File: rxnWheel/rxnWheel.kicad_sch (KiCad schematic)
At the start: 14 parts, among them IC1 TB9061AFNG,EL

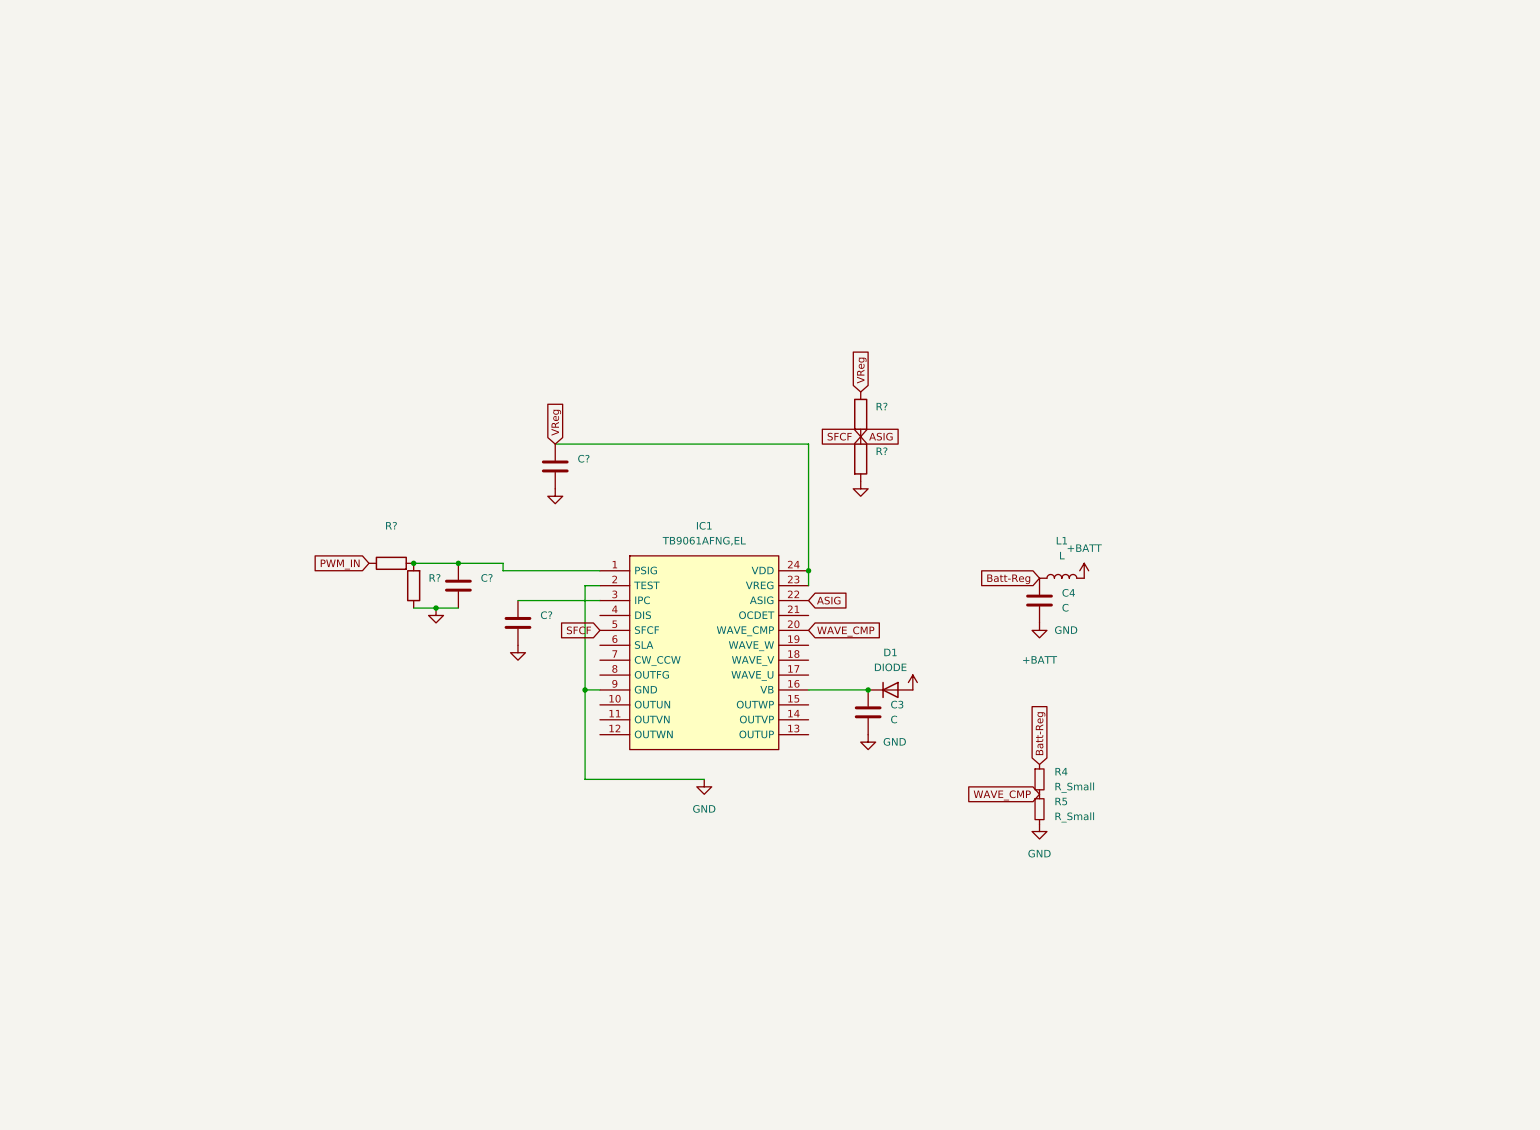
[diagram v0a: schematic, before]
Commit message: .
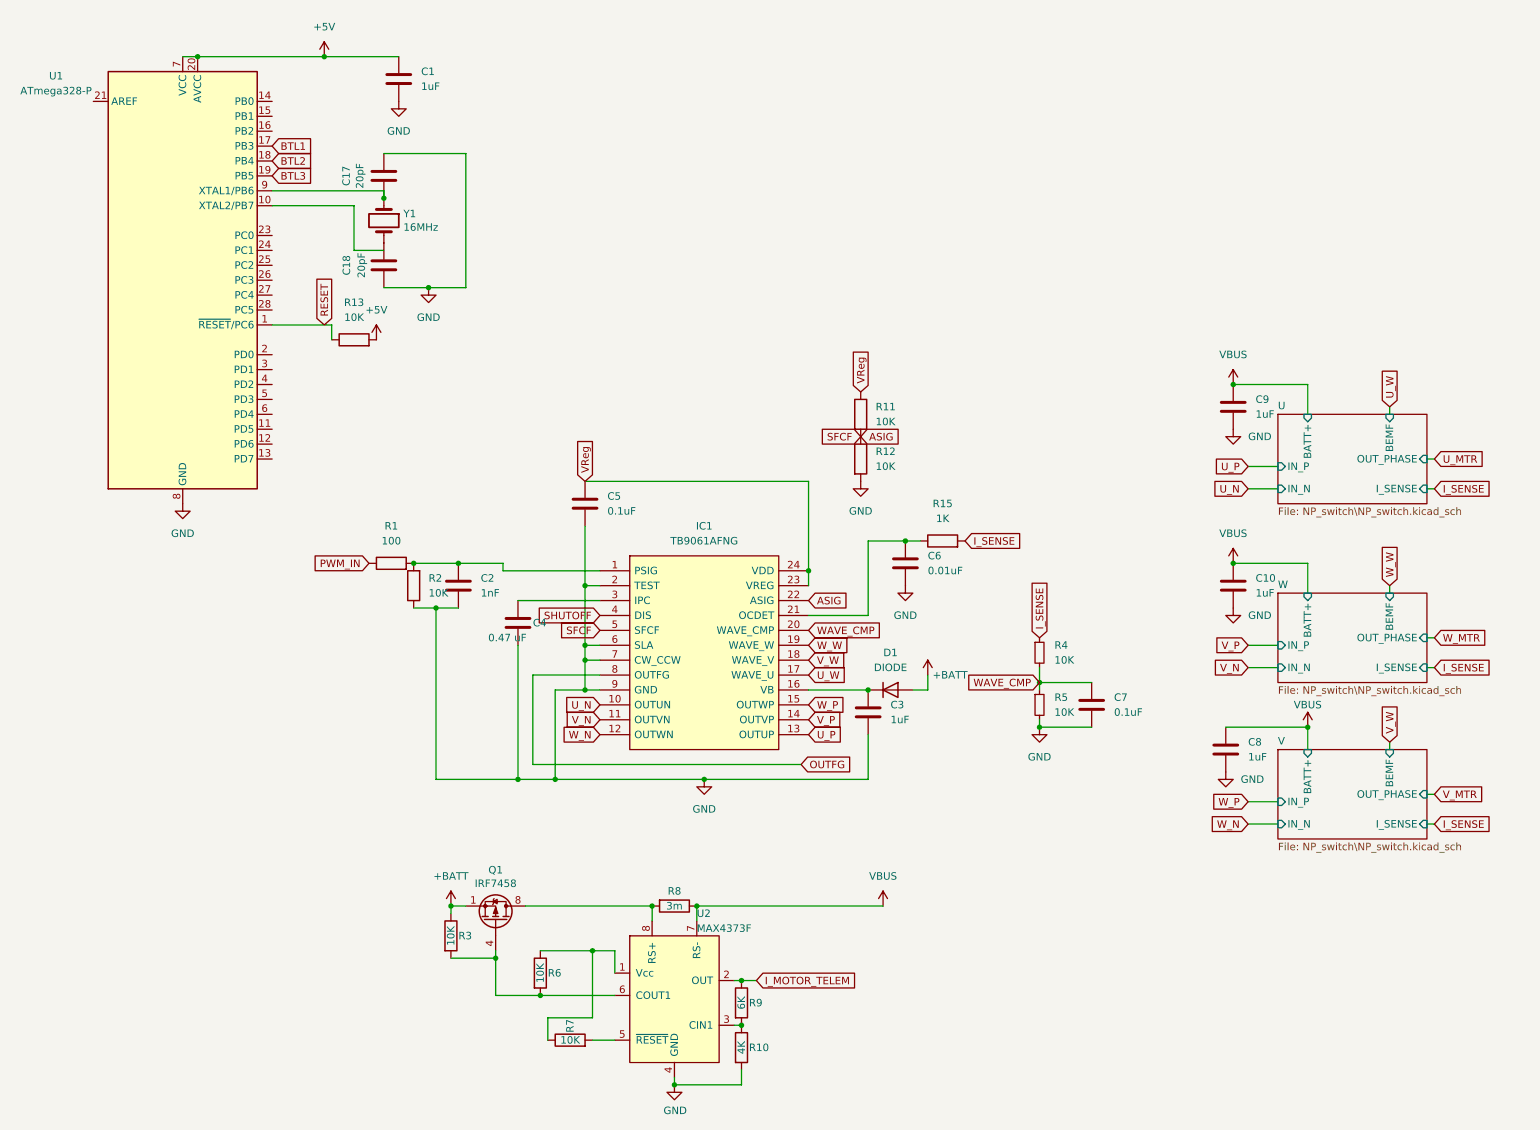
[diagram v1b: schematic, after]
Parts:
- removed C4: C, symbol Device:C
- removed L1: L, symbol Device:L
- added C1, C10, C8, C9: 1uF, Capacitor_SMD:C_0805_2012Metric, symbol Device:C
- added C17, C18: 20pF, Capacitor_SMD:C_0805_2012Metric, symbol Device:C
- added C6: 0.01uF, Capacitor_SMD:C_0805_2012Metric, symbol Device:C
- added C7: 0.1uF, Capacitor_SMD:C_0805_2012Metric, symbol Device:C
- added Q1: IRF7458, Package_SO:SOIC-8_3.9x4.9mm_P1.27mm, symbol Transistor_FET:IRF7404
- added R10: 4K, Resistor_SMD:R_0805_2012Metric, symbol Device:R
- added R13, R3, R6, R7: 10K, Resistor_SMD:R_0805_2012Metric, symbol Device:R
- added R15: 1K, Resistor_SMD:R_0805_2012Metric, symbol Device:R
- added R8: 3m, Resistor_SMD:R_1206_3216Metric, symbol Device:R
- added R9: 6K, Resistor_SMD:R_0805_2012Metric, symbol Device:R
- added U1: ATmega328-P, Package_DIP:DIP-28_W7.62mm, symbol MCU_Microchip_ATmega:ATmega328-P
- added U2: MAX4373F, Package_SO:SO-8_3.9x4.9mm_P1.27mm, symbol symbols:MAX4373F
- added Y1: 16MHz, Crystal:Crystal_HC49-4H_Vertical, symbol Device:Crystal
- C2: renamed from C?; value (none) -> 1nF; footprint (none) -> Capacitor_SMD:C_0805_2012Metric
- C3: value C -> 1uF; footprint (none) -> Capacitor_SMD:C_0805_2012Metric
- C4: renamed from C?; value (none) -> 0.47 uF; footprint (none) -> Capacitor_SMD:C_0805_2012Metric
- C5: renamed from C?; value (none) -> 0.1uF; footprint (none) -> Capacitor_SMD:C_0805_2012Metric
- IC1: value TB9061AFNG,EL -> TB9061AFNG; footprint SOP65P760X160-24N -> TB9061AFNG:SOP65P760X160-24N
- R1: renamed from R?; value (none) -> 100; footprint (none) -> Resistor_SMD:R_0805_2012Metric
- R11, R12, R2: renamed from R?; value (none) -> 10K; footprint (none) -> Resistor_SMD:R_0805_2012Metric
- R4, R5: value R_Small -> 10K; footprint (none) -> Resistor_SMD:R_0805_2012Metric
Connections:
- net +BATT: now also Q1.1 (S), Q1.2 (S), Q1.3 (S), R3.1
- net GND: now also IC1.6 (SLA), IC1.7 (CW_CCW), C1.2, C10.2, C17.1, C18.1, C6.1, C7.1, C8.2, C9.2, R10.2, U1.22 (GND), U1.8 (GND), U2.4 (GND)
- net WAVE_CMP: now also C7.2
- net U_N: now reaches IC1.10 (OUTUN)
- net V_N: now reaches IC1.11 (OUTVN)
- net W_N: now reaches IC1.12 (OUTWN)
- net U_P: now reaches IC1.13 (OUTUP)
- net V_P: now reaches IC1.14 (OUTVP)
- net W_P: now reaches IC1.15 (OUTWP)
- net U_W: now reaches IC1.17 (WAVE_U)
- net V_W: now reaches IC1.18 (WAVE_V)
- net W_W: now reaches IC1.19 (WAVE_W)
- net at IC1.21 (OCDET): now also C6.2, R15.1
- net SHUTOFF: now reaches IC1.4 (DIS)
- net OUTFG: now reaches IC1.8 (OUTFG)
- net Batt-Reg renamed I_SENSE
- net I_SENSE: now also R15.2
- new net: Q1.4 (G), R3.2, R6.2, U2.6 (COUT1)
- new net: Q1.5 (D), Q1.6 (D), Q1.7 (D), Q1.8 (D), R8.2, U2.8 (RS+)
- new net: R6.1, R7.1, U2.1 (Vcc)
- new net: R7.2, U2.5 (~{RESET})
- new net: C18.2, Y1.2
- new net: R10.1, R9.2, U2.3 (CIN1)
- new net: C17.2, U1.9 (XTAL1/PB6), Y1.1
- new net +5V: C1.1, R13.2, U1.20 (AVCC), U1.7 (VCC)
- new net BTL1: U1.17 (PB3)
- new net BTL2: U1.18 (PB4)
- new net BTL3: U1.19 (PB5)
- new net I_MOTOR_TELEM: R9.1, U2.2 (OUT)
- new net RESET: R13.1, U1.1 (~{RESET}/PC6)
- new net VBUS: C10.1, C8.1, C9.1, R8.1, U2.7 (RS-)
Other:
- added sheet U (NP_switch\NP_switch.kicad_sch)
- added sheet V (NP_switch\NP_switch.kicad_sch)
- added sheet W (NP_switch\NP_switch.kicad_sch)
- moved on the sheet: C5, R4, R5

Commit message: Commit
CoMmMMmMMMmits
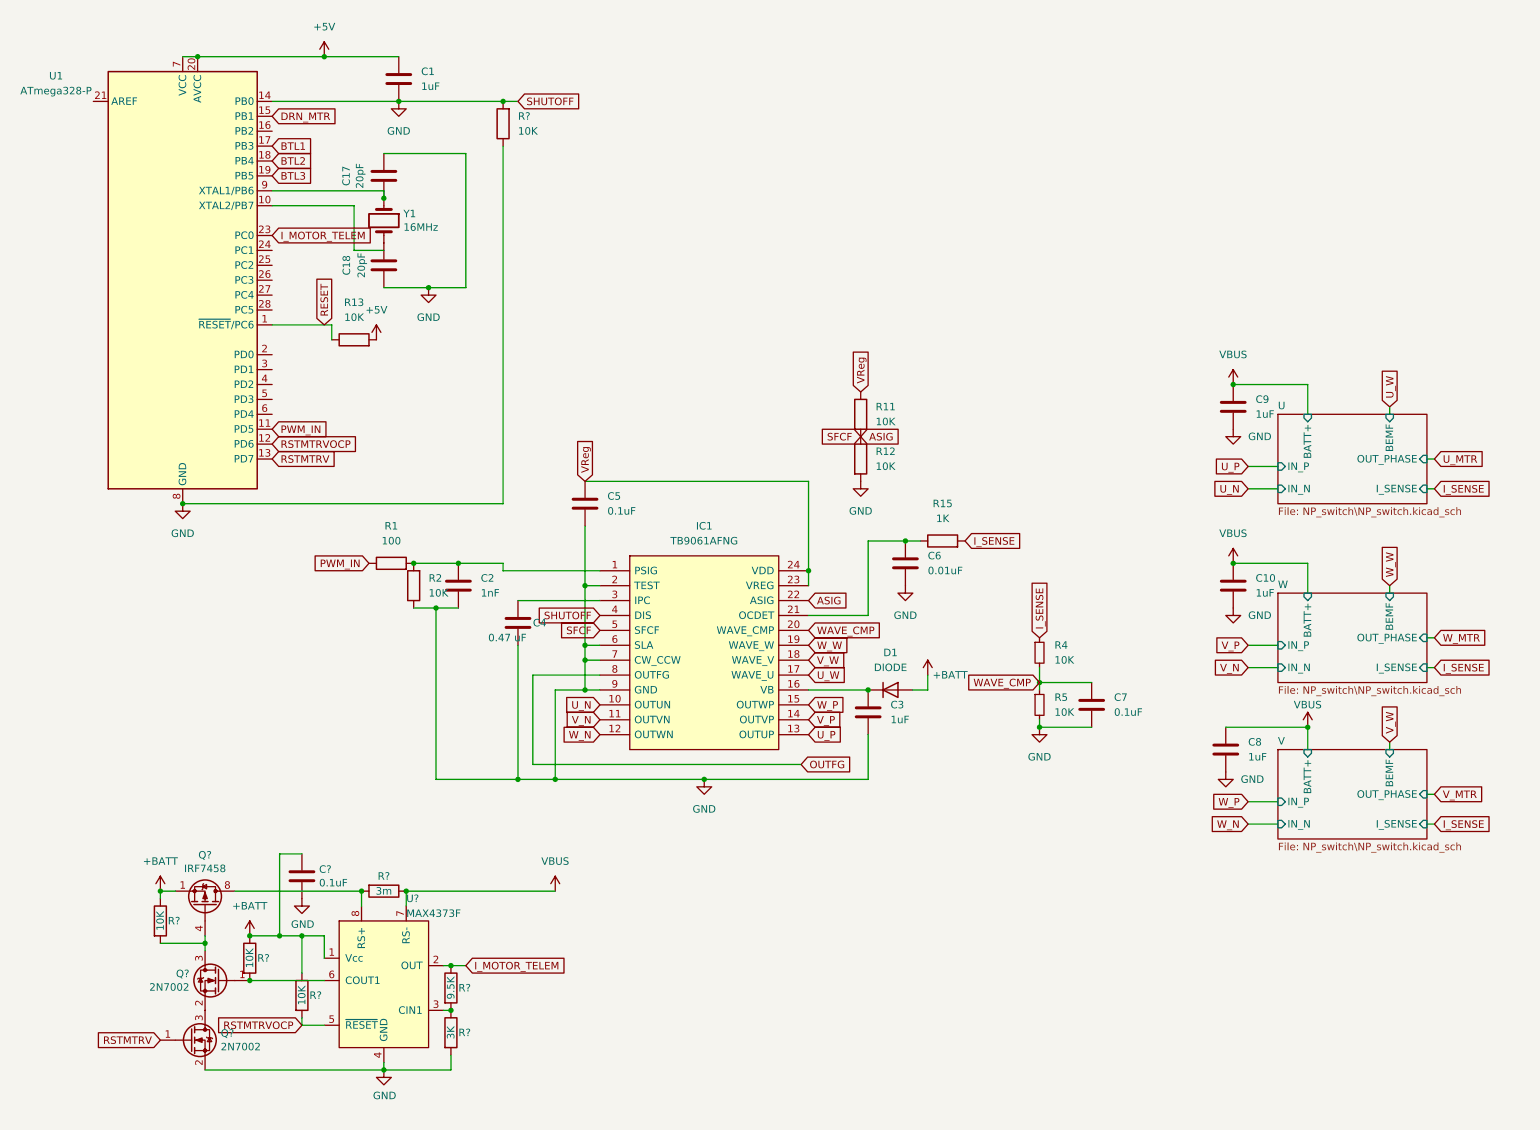
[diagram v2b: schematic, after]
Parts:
- removed Q1: IRF7458, Package_SO:SOIC-8_3.9x4.9mm_P1.27mm, symbol Transistor_FET:IRF7404
- removed R10: 4K, Resistor_SMD:R_0805_2012Metric, symbol Device:R
- removed R3, R6, R7: 10K, Resistor_SMD:R_0805_2012Metric, symbol Device:R
- removed R8: 3m, Resistor_SMD:R_1206_3216Metric, symbol Device:R
- removed R9: 6K, Resistor_SMD:R_0805_2012Metric, symbol Device:R
- removed U2: MAX4373F, Package_SO:SO-8_3.9x4.9mm_P1.27mm, symbol symbols:MAX4373F
- added C?: 0.1uF, Capacitor_SMD:C_0805_2012Metric, symbol Device:C
- added Q? (x2): 2N7002, Package_TO_SOT_SMD:SOT-23, symbol Transistor_FET:2N7002
- added Q?: IRF7458, Package_SO:SOIC-8_3.9x4.9mm_P1.27mm, symbol Transistor_FET:IRF7404
- added R? (x4): 10K, Resistor_SMD:R_0805_2012Metric, symbol Device:R
- added R?: 3m, Resistor_SMD:R_1206_3216Metric, symbol Device:R
- added R?: 3K, Resistor_SMD:R_0805_2012Metric, symbol Device:R
- added R?: 9.5K, Resistor_SMD:R_0805_2012Metric, symbol Device:R
- added U?: MAX4373F, Package_SO:SO-8_3.9x4.9mm_P1.27mm, symbol symbols:MAX4373F
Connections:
- net SHUTOFF is gone; now on net GND: IC1.4 (DIS)
- net +BATT: now also C?.1, Q?.1 (S), Q?.2 (S), Q?.3 (S), R?.1, R?.1, R?.1, U?.1 (Vcc)
- net GND: now also U1.14 (PB0), C?.2, Q?.2 (S), R?.1, R?.2, R?.2, U?.4 (GND)
- net I_MOTOR_TELEM: now also U1.23 (PC0), R?.1, U?.2 (OUT)
- net PWM_IN: now also U1.11 (PD5)
- net VBUS: now also R?.1, U?.7 (RS-)
- net RSTMTRVOCP: now reaches U1.12 (PD6)
- net RSTMTRVOCP: now also R?.2, U?.5 (~{RESET})
- net RSTMTRV: now reaches U1.13 (PD7)
- net RSTMTRV: now also Q?.1 (G)
- net DRN_MTR: now reaches U1.15 (PB1)
- new net: Q?.2 (S), Q?.3 (D)
- new net: R?.1, R?.2, U?.3 (CIN1)
- new net: Q?.1 (G), R?.2, U?.6 (COUT1)
- new net: Q?.5 (D), Q?.6 (D), Q?.7 (D), Q?.8 (D), R?.2, U?.8 (RS+)
- new net: Q?.3 (D), Q?.4 (G), R?.2

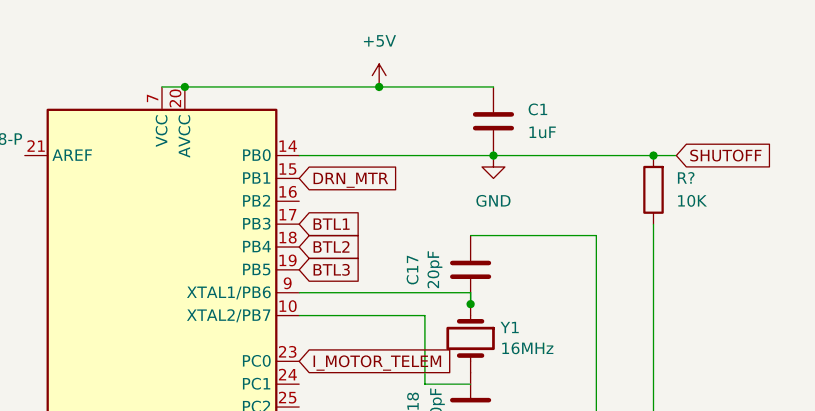
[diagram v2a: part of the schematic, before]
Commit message: HANDS
fix fix hands hands
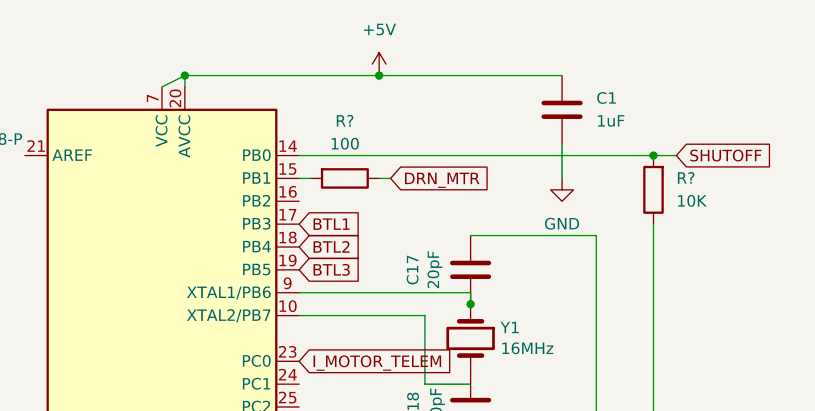
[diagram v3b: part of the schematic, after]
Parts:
- added R?: 100, Resistor_SMD:R_0805_2012Metric, symbol Device:R
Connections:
- net DRN_MTR: now also R?.1; no longer U1.15 (PB1)
- net GND: no longer IC1.4 (DIS), R?.2, U1.14 (PB0)
- new net: R?.2, U1.15 (PB1)
- new net SHUTOFF: IC1.4 (DIS), R?.2, U1.14 (PB0)
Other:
- moved on the sheet: C1
